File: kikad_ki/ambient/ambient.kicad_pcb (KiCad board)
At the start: 2 copper layers, 80 x 66 mm, 69 parts, among them J1 5V DC, J2 FPC 01x10 Female, J3 LED Array, Q1 2N3904, SW1 Reset, SW2 Next, SW3 Select, SW4 Modify, U1 ATmega328P-PU, U2 AT24C256, U3 AT24C256, U4 AT24C256, U5 AT24C256, Y1 16 MHz

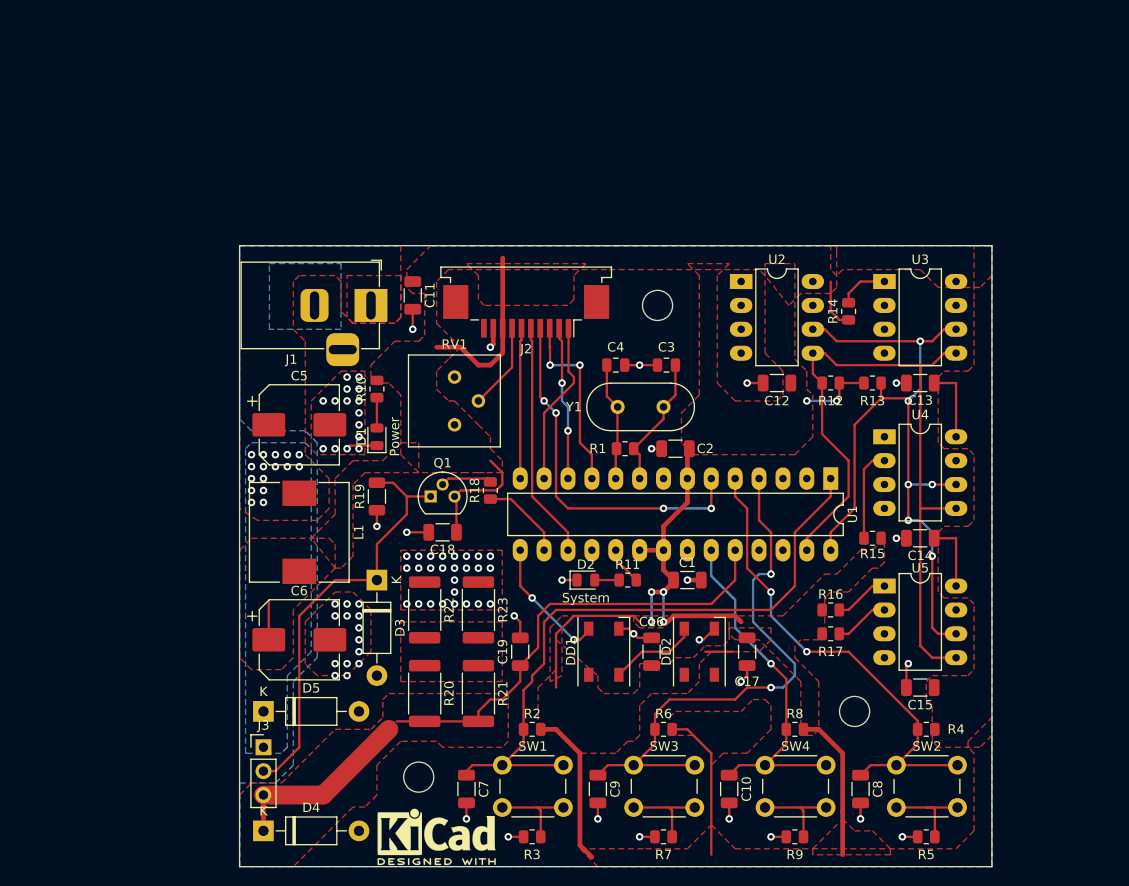
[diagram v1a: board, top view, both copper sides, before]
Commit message: updated design + pcb
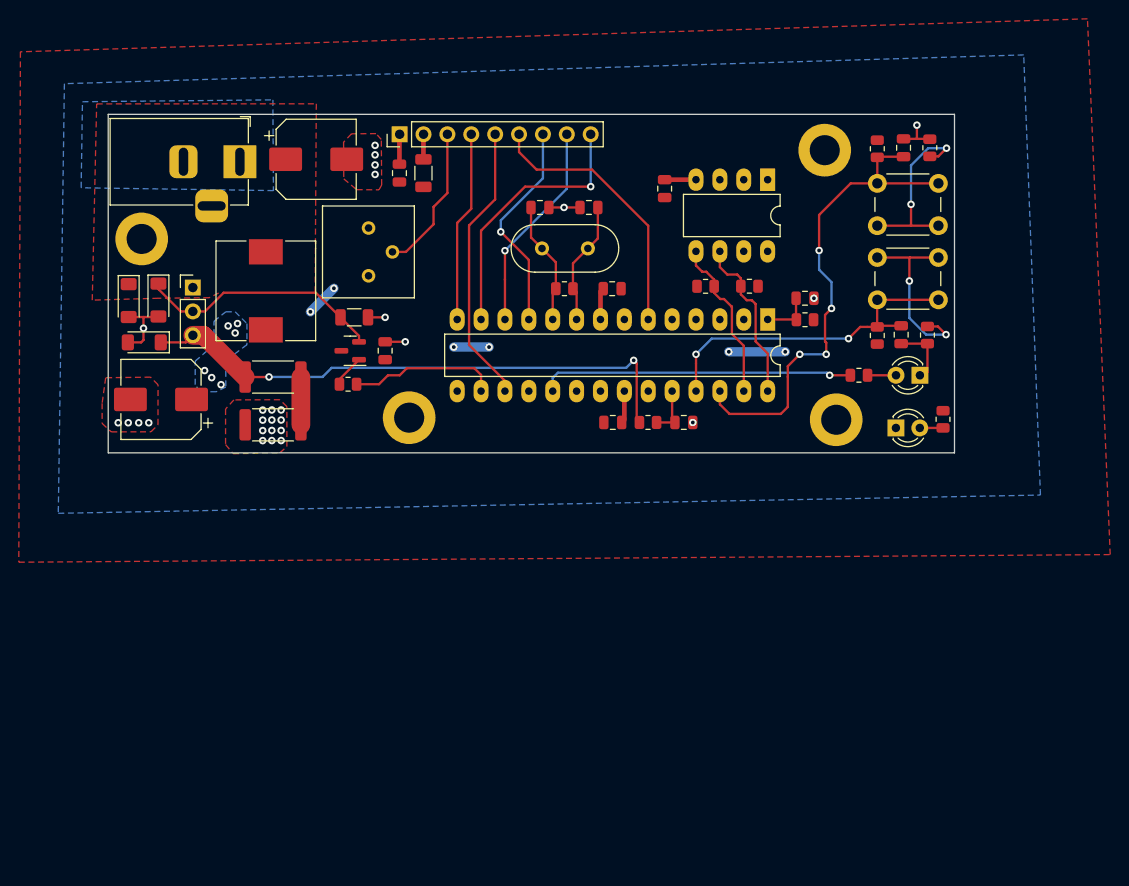
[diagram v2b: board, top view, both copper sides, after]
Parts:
- removed  : MountingHole_3.2mm_M3, MountingHole:MountingHole_3.2mm_M3 (x3)
- removed the C13 at (86.4, 28.6)
- removed C14, C15, C16, C17, C19: 0.1u, Capacitor_SMD:C_1206_3216Metric
- removed the C3 at (59.4, 26.7)
- removed D4, D5: 1N4735A, Diode_THT:D_DO-41_SOD81_P10.16mm_Horizontal
- removed DD1, DD2: SK6812, LED_SMD:LED_SK6812_PLCC4_5.0x5.0mm_P3.2mm
- removed R14, R15, R16, R17: 4.7k, Resistor_SMD:R_0805_2012Metric
- removed R22, R23: 0.02, Resistor_SMD:R_2512_6332Metric
- removed R9: 68, Resistor_SMD:R_0805_2012Metric
- removed the SW1 at (41.9, 69.2)
- removed SW4: Modify, Button_Switch_THT:SW_PUSH_6mm
- removed U3, U4, U5: AT24C256, Package_DIP:DIP-8_W7.62mm_LongPads
- added ?: , rasp:prv_small, B.Cu at (17.2, 14.8)
- added C6: 22, Capacitor_SMD:C_0805_2012Metric, F.Cu at (51.1, 9.91)
- added H1: MountingHole, MountingHole:MountingHole_3.2mm_M3_DIN965_Pad, F.Cu at (3.56, 13.2)
- added H2: MountingHole, MountingHole:MountingHole_3.2mm_M3_DIN965_Pad, F.Cu at (32.0, 32.3)
- added H3: MountingHole, MountingHole:MountingHole_3.2mm_M3_DIN965_Pad, F.Cu at (76.2, 3.81)
- added H4: MountingHole, MountingHole:MountingHole_3.2mm_M3_DIN965_Pad, F.Cu at (77.4, 32.5)
- added LED1: Blue LED, LED_THT:LED_D3.0mm_Clear, F.Cu at (86.3, 27.8)
- added LED2: Green LED, LED_THT:LED_D3.0mm_Clear, F.Cu at (83.8, 33.4)
- C1: renamed from C6; value 330u 16V -> 100u 25V
- C10: footprint Capacitor_SMD:C_1206_3216Metric -> Capacitor_SMD:C_0805_2012Metric
- C11: renamed from C7; footprint Capacitor_SMD:C_1206_3216Metric -> Capacitor_SMD:C_0805_2012Metric
- C12: renamed from C8; footprint Capacitor_SMD:C_1206_3216Metric -> Capacitor_SMD:C_0805_2012Metric
- C13: renamed from C9; footprint Capacitor_SMD:C_1206_3216Metric -> Capacitor_SMD:C_0805_2012Metric
- C2: renamed from C5; value 330u 16V -> 100u 25V
- C3: renamed from C18; footprint Capacitor_SMD:C_1206_3216Metric -> Capacitor_SMD:C_0805_2012Metric
- C4: renamed from C11; footprint Capacitor_SMD:C_1206_3216Metric -> Capacitor_SMD:C_0805_2012Metric
- C7: renamed from C2; footprint Capacitor_SMD:C_1206_3216Metric -> Capacitor_SMD:C_0805_2012Metric
- C8: renamed from C1; footprint Capacitor_SMD:C_1206_3216Metric -> Capacitor_SMD:C_0805_2012Metric
- C9: renamed from C12; footprint Capacitor_SMD:C_1206_3216Metric -> Capacitor_SMD:C_0805_2012Metric
- D1: value Green LED -> 1N4735A; footprint LED_SMD:LED_0805_2012Metric -> Diode_SMD:D_MiniMELF
- D2: value Blue LED -> 1N4735A; footprint LED_SMD:LED_0805_2012Metric -> Diode_SMD:D_MiniMELF
- D3: footprint Diode_THT:D_DO-41_SOD81_P10.16mm_Horizontal -> Diode_SMD:D_MiniMELF
- J2: value FPC 01x10 Female -> Display; footprint Connector_FFC-FPC:TE_1-84952-0_1x10-1MP_P1.0mm_Horizontal -> Connector_PinHeader_2.54mm:PinHeader_1x09_P2.54mm_Vertical
- L1: value 100u -> 47u
- Q1: value 2N3904 -> MMBT3904; footprint Package_TO_SOT_THT:TO-92 -> Package_TO_SOT_SMD:SOT-23
- R10: value 3k -> 2k
- R11: value 3k -> 1k
- R2: value 5.1k -> 10k
- R3: value 68 -> 100; footprint Resistor_SMD:R_0805_2012Metric -> Resistor_SMD:R_1206_3216Metric
- R5, R7: value 68 -> 200
- R8: value 5.1k -> 100k
- REF**: moved to B.Cu
- moved R5 73.3 mm to (87.4, 3.56), turned to -90 degrees
- moved R3 71.5 mm to (33.5, 6.25), turned to -90 degrees
- moved REF** 70.0 mm to (35.8, 6.84), turned to 180 degrees
- moved C12 68.4 mm to (84.6, 3.56), turned to 90 degrees
- moved C11 63.4 mm to (74.1, 19.6), turned to 0 degrees
- moved R4 62.0 mm to (81.8, 3.66), turned to 90 degrees
- moved SW1 61.9 mm to (81.8, 7.34)
- moved R7 60.3 mm to (87.1, 23.5), turned to 90 degrees
- moved R10 60.3 mm to (88.8, 32.4)
- moved SW2 59.2 mm to (88.3, 19.7), turned to 180 degrees
- moved C13 58.1 mm to (84.3, 23.4)
- moved D2 54.3 mm to (5.34, 19.8), turned to -90 degrees
- moved R2 52.3 mm to (74.1, 21.8)
- moved J3 49.5 mm to (9.00, 18.4)
- moved R6 47.7 mm to (81.8, 23.5), turned to -90 degrees
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- renumbered C4 to C5, SW2 to SW1, SW3 to SW2
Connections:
- C10 pad 1: MODIFY -> AMP_IN
- C12 pad 1: NEXT -> MODE
- D1 pad 1: GND -> +5V
- D1 pad 2: Net-(D1-Pad2) -> GND
- D2 pad 1: GND -> ARRAY_DIN
- D2 pad 2: Net-(D2-Pad2) -> GND
- D3 pad 1: ARRAY_DIN -> ARRAY_GND
- J2 pad 1: LCD_DB7 -> GND
- J2 pad 2: LCD_DB6 -> Net-(J2-Pin_2)
- J2 pad 3: LCD_DB5 -> Net-(J2-Pin_3)
- J2 pad 4: LCD_DB4 -> LCD_RS
- J2 pad 6: LCD_RS -> LCD_DB4
- J2 pad 7: Net-(J2-Pad7) -> LCD_DB5
- J2 pad 8: VCC -> LCD_DB6
- J2 pad 9: GND -> LCD_DB7
- J3 pad 3: AMP_IN -> ARRAY_GND
- Q1 pad 1: ARRAY_DIN -> Net-(Q1-B)
- Q1 pad 2: Net-(Q1-Pad2) -> ARRAY_DIN
- R10 pad 1: Net-(D1-Pad2) -> Net-(LED2-A)
- R11 pad 1: Net-(D2-Pad2) -> Net-(LED1-A)
- R18 pad 2: Net-(Q1-Pad2) -> Net-(Q1-B)
- R20 pad 2: AMP_IN -> ARRAY_GND
- R21 pad 1: Net-(R20-Pad1) -> GND
- R21 pad 2: AMP_IN -> Net-(R20-Pad1)
- R3 pad 1: GND -> Net-(J2-Pin_2)
- R3 pad 2: Net-(R3-Pad2) -> VCC
- R4 pad 1: NEXT -> MODE
- R8 pad 1: MODIFY -> ARRAY_GND
- R8 pad 2: VCC -> AMP_IN
- RV1 pad 2: Net-(J2-Pad7) -> Net-(J2-Pin_3)
- SW1 pad 1: NEXT -> MODE
- U1 pad 15: PREVIEW_ARRAY -> unconnected-(U1-PB1-Pad15)
- U1 pad 18: Net-(U1-Pad18) -> unconnected-(U1-PB4-Pad18)
- U1 pad 2: Net-(U1-Pad2) -> unconnected-(U1-PD0-Pad2)
- U1 pad 23: MODIFY -> unconnected-(U1-PC0-Pad23)
- U1 pad 25: Net-(U1-Pad25) -> SELECT
- U1 pad 26: Net-(U1-Pad26) -> MODE
- U1 pad 3: Net-(U1-Pad3) -> unconnected-(U1-PD1-Pad3)
- U1 pad 4: SELECT -> unconnected-(U1-PD2-Pad4)
- U1 pad 5: NEXT -> unconnected-(U1-PD3-Pad5)
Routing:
- net VCC: track 168.5 -> 13.3 mm, vias 6 -> 12
- net RESET: track 69.3 -> 5.32 mm
- net AMP_IN: track 69.0 -> 5.40 mm
- net SCL: track 80.6 -> 17.9 mm, vias 6 -> 0
- net SDA: track 79.5 -> 17.5 mm
- net ARRAY_GND: track 0.00 -> 60.1 mm, vias 0 -> 2
- net MODE: track 0.00 -> 53.7 mm, vias 0 -> 4
- net NEXT: track 52.8 -> 0.00 mm, vias 2 -> 0
- net MODIFY: track 37.9 -> 0.00 mm, vias 1 -> 0
- net LED: track 4.08 -> 33.4 mm, vias 0 -> 1
- net SELECT: track 58.6 -> 36.4 mm
- net ARRAY_DIN: track 45.2 -> 26.3 mm
- net Net-(J2-Pin_3): track 0.00 -> 15.8 mm
- net PREVIEW_ARRAY: track 14.2 -> 0.00 mm, vias 2 -> 0
- net GND: track 50.7 -> 39.2 mm, vias 79 -> 27
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- added copper zone on B.Cu, net VCC
- removed copper zone on B.Cu, net +5V
- removed copper zone on F.Cu, net AMP_IN
- removed copper zone on F.Cu, net Net-(R20-Pad1)
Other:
- board size 80 x 66 mm -> 90 x 36 mm
- net class Default removed
- board text added: "JLCJLCJLCJLC"
- board text removed: "Power"
- board text removed: "System"
